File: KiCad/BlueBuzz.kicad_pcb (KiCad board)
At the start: 2 copper layers, 19.5 x 25.2 mm, 11 parts, among them J1 Conn_01x06_Socket, J2 DE9, SW1 SW_DIP_x01, SW2 SW_DIP_x01, U1 ESP32, U2 AMS1117

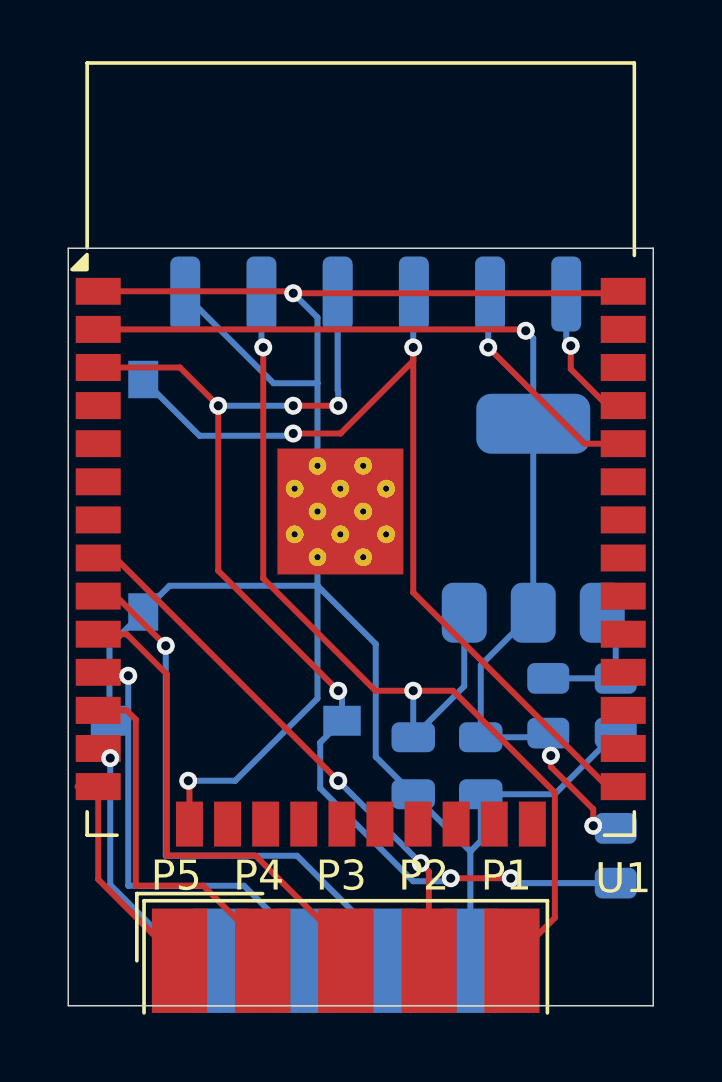
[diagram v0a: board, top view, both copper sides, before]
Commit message: update PCB
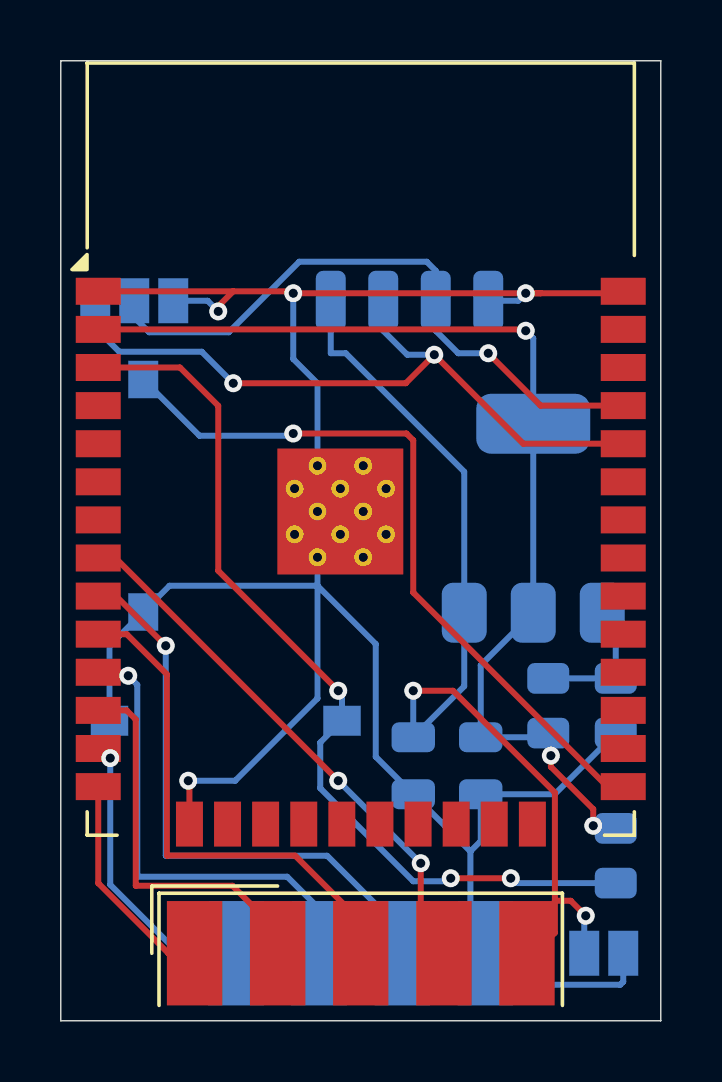
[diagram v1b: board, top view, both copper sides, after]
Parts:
- added J0: DE9, Connector_Dsub:DSUB-9_Pins_EdgeMount_P2.77mm, F.Cu at (154.8, 85.8)
- added J3: Conn_01x03_Socket, Jumper:SolderJumper-3_P1.3mm_Open_Pad1.0x1.5mm_NumberLabels, B.Cu at (147.2, 64.0)
- added J4: Conn_01x02_Socket, Jumper:SolderJumper-2_P1.3mm_Open_Pad1.0x1.5mm, B.Cu at (162.8, 85.8)
- added J5: Conn_01x01_Socket, Connector_Wire:SolderWirePad_1x01_SMD_1x2mm, B.Cu at (153.8, 64.0)
- added J6: Conn_01x01_Socket, Connector_Wire:SolderWirePad_1x01_SMD_1x2mm, B.Cu at (159.0, 64.0)
- J1: value Conn_01x06_Socket -> Conn_01x01_Socket; footprint Connector_Harwin:Harwin_M20-89006xx_1x06_P2.54mm_Horizontal -> Connector_Wire:SolderWirePad_1x01_SMD_1x2mm
- J2: value DE9 -> Conn_01x01_Socket; footprint Connector_Dsub:DSUB-9_Pins_EdgeMount_P2.77mm -> Connector_Wire:SolderWirePad_1x01_SMD_1x2mm; moved to B.Cu
- moved J2 22.0 mm to (155.5, 64.0), turned to 180 degrees
- moved J1 6.09 mm to (157.2, 64.0), turned to 180 degrees
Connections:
- C1 pad 1: Net-(J1-Pin_6) -> Net-(J3-Pin_1)
- C1 pad 2: Net-(J1-Pin_5) -> Net-(J4-Pin_2)
- C2 pad 1: Net-(J1-Pin_6) -> Net-(J3-Pin_1)
- J2 pad 1: Net-(U1-IO12) -> Net-(J2-Pin_1)
- R2 pad 2: Net-(J1-Pin_6) -> Net-(J3-Pin_1)
- R3 pad 2: Net-(J1-Pin_4) -> Net-(U1-EN)
- SW1 pad 1: Net-(J1-Pin_3) -> Net-(U1-IO0)
- SW1 pad 2: Net-(J1-Pin_6) -> Net-(J3-Pin_1)
- SW2 pad 1: Net-(J1-Pin_4) -> Net-(U1-EN)
- SW2 pad 2: Net-(J1-Pin_6) -> Net-(J3-Pin_1)
- U1 pad 1: Net-(J1-Pin_6) -> Net-(J3-Pin_1)
- U1 pad 15: Net-(J1-Pin_6) -> Net-(J3-Pin_1)
- U1 pad 25: Net-(J1-Pin_3) -> Net-(U1-IO0)
- U1 pad 3: Net-(J1-Pin_4) -> Net-(U1-EN)
- U1 pad 34: Net-(J1-Pin_2) -> Net-(J2-Pin_1)
- U1 pad 38: Net-(J1-Pin_6) -> Net-(J3-Pin_1)
- U1 pad 39: Net-(J1-Pin_6) -> Net-(J3-Pin_1)
- U2 pad 3: Net-(J1-Pin_5) -> Net-(J4-Pin_2)
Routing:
- net Net-(J3-Pin_1): track 0.00 -> 81.7 mm, vias 0 -> 4
- net Net-(J1-Pin_6): track 76.9 -> 0.00 mm, vias 2 -> 0
- net Net-(J1-Pin_4): track 37.8 -> 0.00 mm, vias 6 -> 0
- net Net-(J1-Pin_5): track 34.8 -> 0.00 mm, vias 2 -> 0
- net Net-(J4-Pin_2): track 0.00 -> 33.2 mm, vias 0 -> 2
- net Net-(J1-Pin_3): track 30.9 -> 0.00 mm, vias 2 -> 0
- net Net-(U1-EN): track 0.00 -> 30.1 mm, vias 0 -> 3
- net Net-(U1-IO0): track 0.00 -> 24.7 mm, vias 0 -> 1
- net Net-(J2-Pin_1): track 0.00 -> 23.9 mm, vias 0 -> 2
- net Net-(J1-Pin_1): track 4.82 -> 21.2 mm
- net Net-(J1-Pin_2): track 7.63 -> 0.00 mm, vias 1 -> 0
- net Net-(U1-IO25): track 16.6 -> 17.4 mm
- net Net-(U1-IO26): track 15.2 -> 16.0 mm
- net Net-(U1-IO33): track 19.1 -> 19.7 mm
- net Net-(U1-IO14): track 9.50 -> 10.1 mm
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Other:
- board size 19.5 x 25.2 mm -> 20 x 32 mm
- board text added: "BuzzLink"
- board text removed: "D0"
- board text removed: "EN"
- board text removed: "P1"
- board text removed: "P2"
- board text removed: "P3"
- board text removed: "P4"
- board text removed: "P5"
